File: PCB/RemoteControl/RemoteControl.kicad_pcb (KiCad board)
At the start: 2 copper layers, 106.8 x 80.3 mm, 24 parts, among them J1 USB_C_Receptacle_USB2.0_14P, J2 Conn_01x02_Pin, J3 Conn_01x05_Pin, J4 Conn_01x02_Socket, J5 Conn_01x06_Socket, J6 Conn_01x02_Socket, J7 Conn_01x02_Socket, J8 Conn_01x02_Socket, J9 Conn_01x02_Socket, U1 STM32L031K6Tx, U2 TC1262-33, U3 NORA-W106-00B

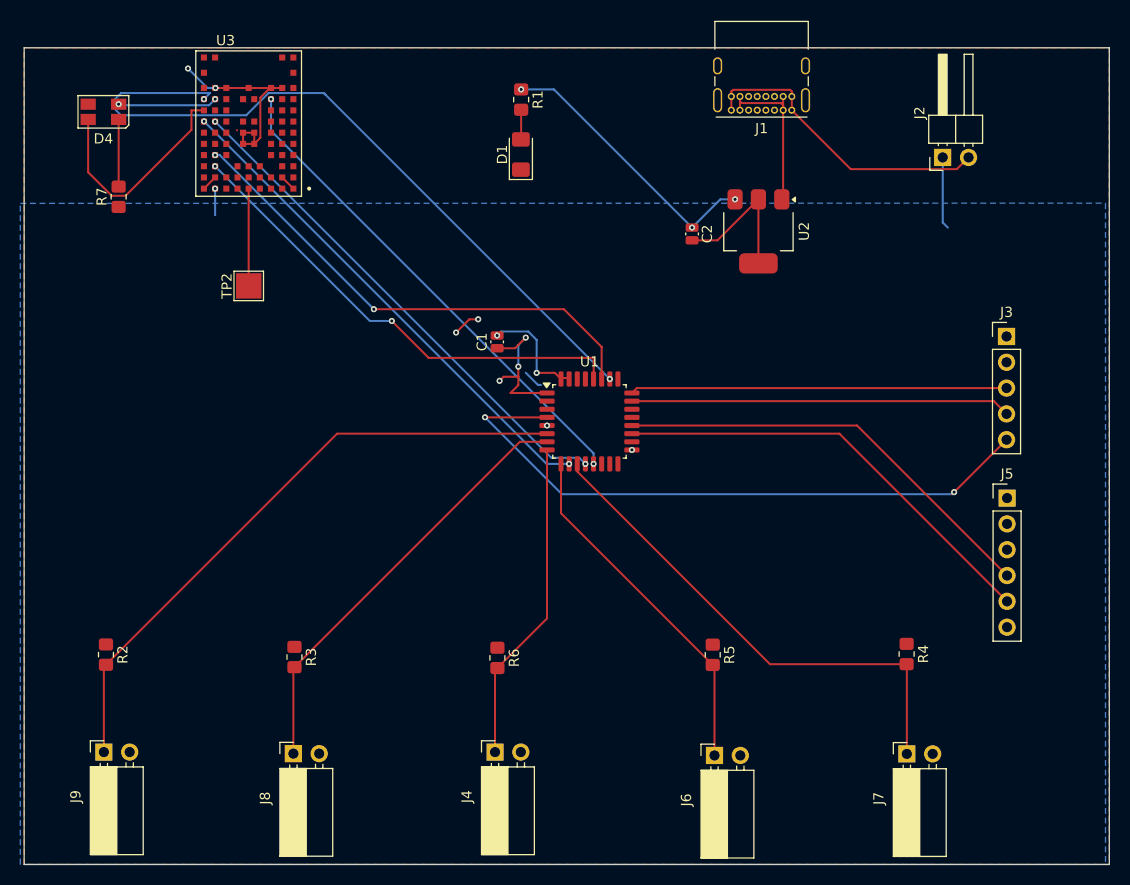
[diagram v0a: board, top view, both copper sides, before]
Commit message: Updated remote control
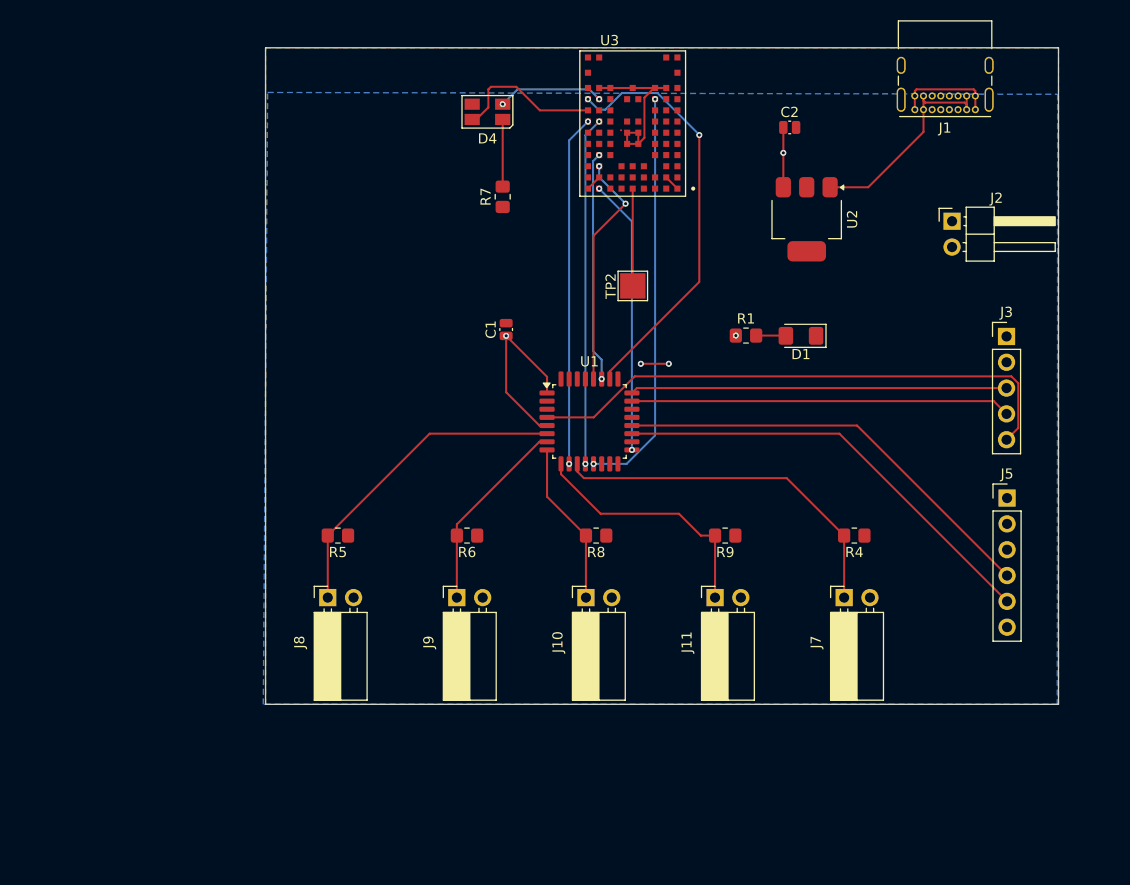
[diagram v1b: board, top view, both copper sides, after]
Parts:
- removed J4, J6: Conn_01x02_Socket, Connector_PinSocket_2.54mm:PinSocket_1x02_P2.54mm_Horizontal
- removed R2, R3: R, Resistor_SMD:R_0805_2012Metric_Pad1.20x1.40mm_HandSolder
- added J10: Conn_01x02_Socket, Connector_PinSocket_2.54mm:PinSocket_1x02_P2.54mm_Horizontal, F.Cu at (123.8, 102.5)
- added J11: Conn_01x02_Socket, Connector_PinSocket_2.54mm:PinSocket_1x02_P2.54mm_Horizontal, F.Cu at (136.6, 102.5)
- added R8: R, Resistor_SMD:R_0805_2012Metric_Pad1.20x1.40mm_HandSolder, F.Cu at (124.8, 96.4)
- added R9: R, Resistor_SMD:R_0805_2012Metric_Pad1.20x1.40mm_HandSolder, F.Cu at (137.6, 96.4)
- moved R5 38.7 mm to (99.5, 96.4), turned to 180 degrees
- moved J9 37.9 mm to (111.2, 102.5)
- moved D4 37.8 mm to (114.2, 54.7)
- moved TP2 37.8 mm to (128.5, 71.8)
- moved R7 37.8 mm to (115.7, 63.1)
- moved U3 37.8 mm to (128.4, 55.9)
- moved D1 32.8 mm to (145.0, 76.8), turned to 180 degrees
- moved R1 32.1 mm to (139.6, 76.7), turned to 0 degrees
- moved J1 18.1 mm to (162.2, 54.5)
- moved J7 16.6 mm to (149.2, 102.5)
- moved J8 15.7 mm to (98.5, 102.5)
- moved C2 14.2 mm to (143.9, 56.2), turned to 0 degrees
- moved R4 12.7 mm to (150.2, 96.4), turned to 180 degrees
- moved R6 12.4 mm to (112.2, 96.4), turned to 180 degrees
- moved J2 6.34 mm to (159.9, 65.5), turned to 0 degrees
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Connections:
- J8 pad 1: Finger2 -> Finger1
- J9 pad 1: Finger1 -> Finger2
- R5 pad 2: Finger4 -> Finger1
- R6 pad 2: Finger3 -> Finger2
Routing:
- net gnd: track 81.3 -> 32.4 mm, vias 4 -> 0
- net GPIO_J9: track 73.4 -> 41.4 mm
- net Finger1: track 61.5 -> 31.8 mm
- net Switch1: track 49.1 -> 22.6 mm
- net Switch2: track 47.1 -> 23.3 mm
- net Finger2: track 42.6 -> 19.4 mm
- net TX: track 50.4 -> 34.2 mm
- net Finger3: track 31.8 -> 16.1 mm
- net RX: track 49.9 -> 34.4 mm
- net Finger5: track 49.8 -> 35.7 mm
- net Finger4: track 34.9 -> 24.8 mm
- net Net-(U1-PA7): track 49.0 -> 40.3 mm
- net NRST: track 63.1 -> 54.3 mm, vias 2 -> 0
- net BlueLED: track 22.2 -> 14.7 mm
- net +5V: track 16.9 -> 22.1 mm
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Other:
- board size 106.8 x 80.3 mm -> 78 x 64.6 mm
